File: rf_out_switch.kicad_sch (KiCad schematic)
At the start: 11 parts, among them P15 CONUFL001-SMD-T, P16 CONUFL001-SMD-T, U33 QPC1022TR7, U34 QPC1022TR7

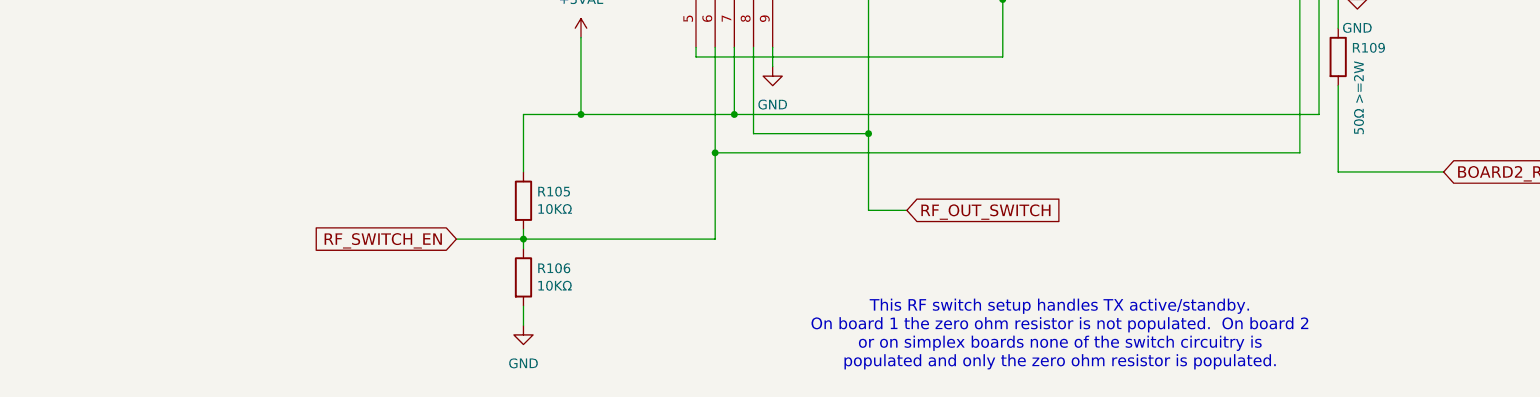
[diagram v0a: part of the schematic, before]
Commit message: Lots of little cleanups
Signed-off-by: Corey Minyard <corey@minyard.net>
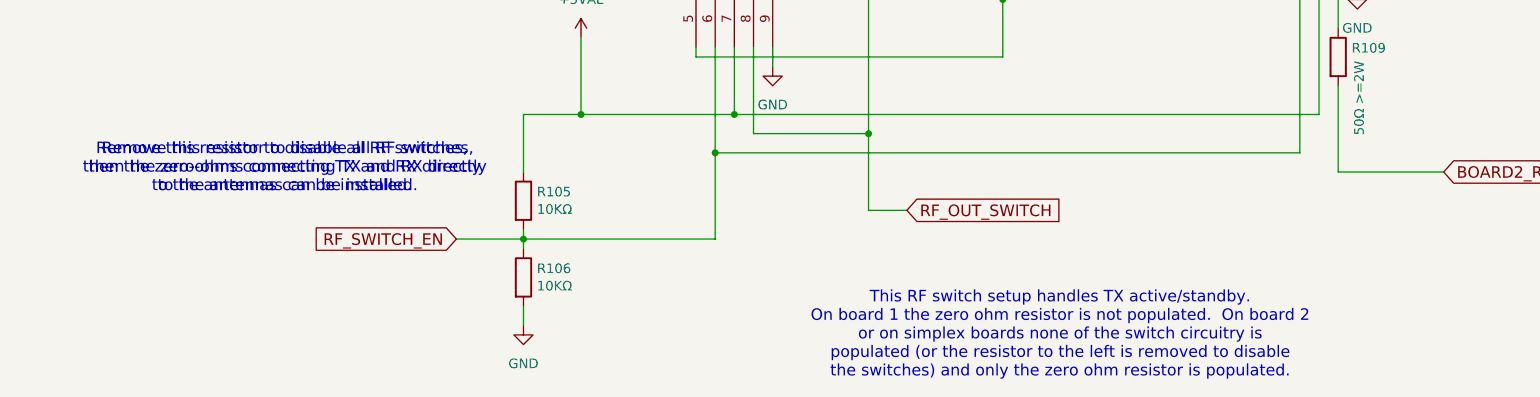
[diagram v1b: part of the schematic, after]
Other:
- note added: "Remove this resistor to disable all RF switches, then the zero-ohms connecting TX and RX directly to the antennas can be installed."
- note added: "This RF switch setup handles TX active/standby. On board 1 the zero ohm resistor is not populated. On board 2 or on simplex boards none of the switch circuitry is populated (or the resistor to the left is removed to disable the switches) and only the zero ohm resistor is populated."
- note removed: "This RF switch setup handles TX active/standby. On board 1 the zero ohm resistor is not populated. On board 2 or on simplex boards none of the switch circuitry is populated and only the zero ohm resistor is populated."
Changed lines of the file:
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@@
 		)
 	)
-	(text "This RF switch setup handles TX active/standby.\nOn board 1 the zero ohm resistor is not populated.  On board 2\nor on simplex boards none of the switch circuitry is\npopulated and only the zero ohm resistor is populated."
+	(text "This RF switch setup handles TX active/standby.\nOn board 1 the zero ohm resistor is not populated.  On board 2\nor on simplex boards none of the switch circuitry is\npopulated (or the resistor to the left is removed to disable\nthe switches) and only the zero ohm resistor is populated."
 		(exclude_from_sim no)
 		(at 156.21 147.32 0)
 		(effects
 			(font
+				(size 1.524 1.524)
+			)
+		)
+	)
+	(text "Remove this resistor to disable all RF switches,\nthen the zero-ohms connecting TX and RX directly\nto the antennas can be installed."
+		(exclude_from_sim no)
+		(at 53.848 125.222 0)
+		(effects
+			(font
+				(size 1.524 1.524)
+			)
+		)
+	)
+	(text "Remove this resistor to disable all RF switches,\nthen the zero-ohms connecting TX and RX directly\nto the antennas can be installed."
+		(exclude_from_sim no)
+		(at 53.086 125.222 0)
+		(effects
+			(font
